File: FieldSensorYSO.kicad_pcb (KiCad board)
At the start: 2 copper layers, 63 x 25 mm, 3 parts, among them J1 22-28-4023, J2 22-28-4023, Y1 Field_Sensor_54_22

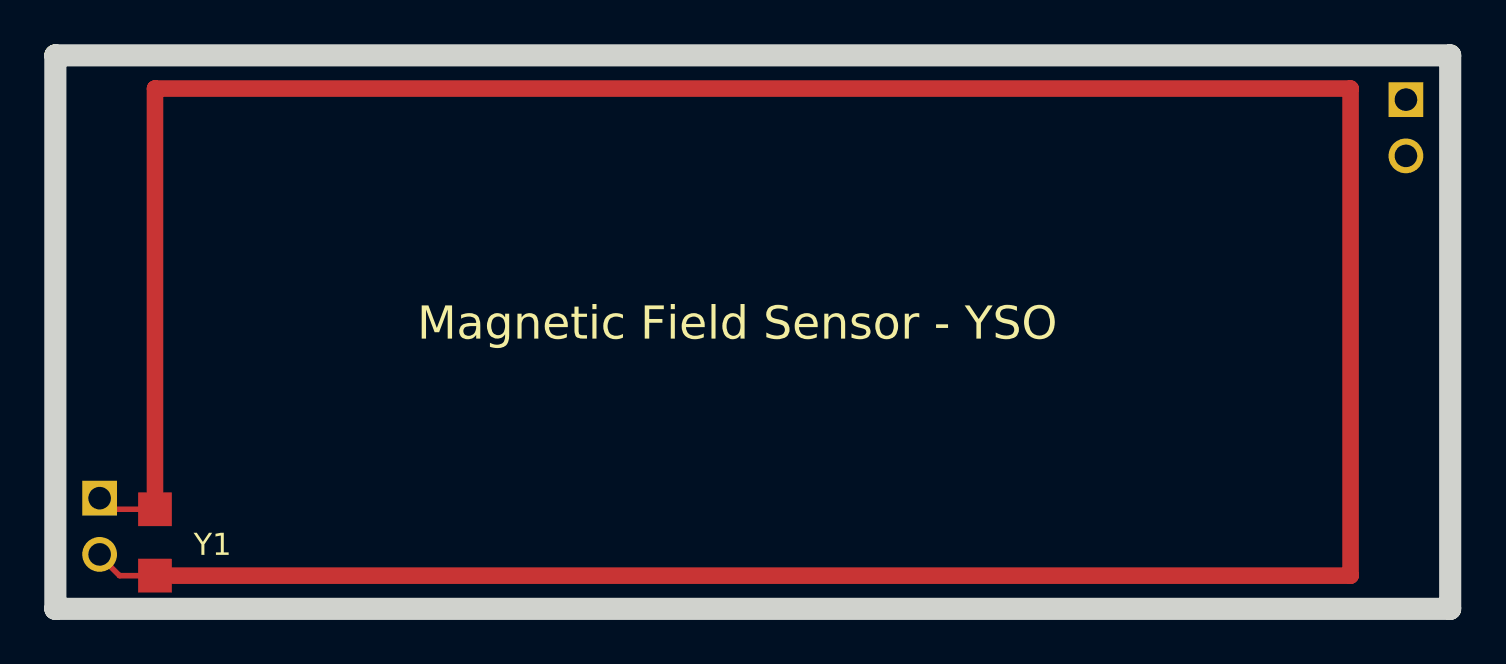
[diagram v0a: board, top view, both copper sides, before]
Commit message: rev 2
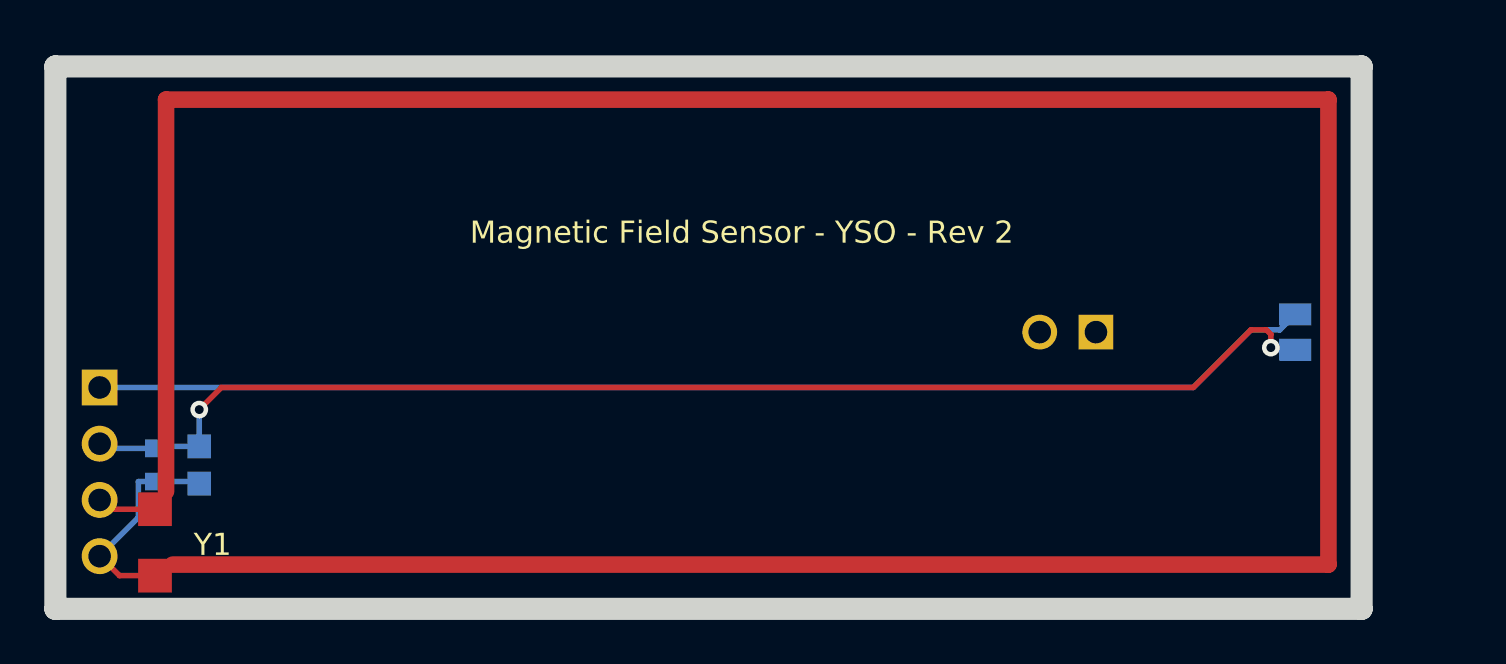
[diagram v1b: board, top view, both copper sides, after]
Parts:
- added C1: CC0603KRX7R9BB102, project:YAGEO-CC0603-0-0-0, B.Cu at (94.5, 108.5)
- added D1: TEMD7000X01, project:XDCR_TEMD7000X01, B.Cu at (146.0, 102.5)
- added R1: RC0603FR-071ML, project:Yageo-RC0603-0-0-IPC_A, B.Cu at (96.5, 108.5)
- J1: value 22-28-4023 -> 22-28-4043; footprint project:Molex-22-28-4023-0-0-0 -> project:Molex-SD-42375-001-0-0-0
- moved J2 17.8 mm to (135.7, 102.5), turned to 180 degrees
- moved J1 2.46 mm to (92.0, 108.8), turned to 180 degrees
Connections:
- J1 pad 1: /HSEN -> /5V
- J1 pad 2: GND -> /LSEN
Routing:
- net /LSEN: track 0.00 -> 58.0 mm, vias 0 -> 2
- net /5V: track 0.00 -> 55.4 mm
- net GND: track 2.87 -> 9.76 mm
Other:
- board size 63 x 25 mm -> 59 x 24.5 mm
- board text added: "Magnetic Field Sensor - YSO - Rev 2"
- board text removed: "Magnetic Field Sensor - YSO"
